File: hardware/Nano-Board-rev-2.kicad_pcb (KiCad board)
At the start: 2 copper layers, 125.7 x 53 mm, 75 parts, among them J1 Conn_01x02_Pin, J2 USB_B_Micro, J3 Conn_02x05_Odd_Even, J4 Conn_02x05_Odd_Even, J5 Conn_02x05_Odd_Even, J6 Micro_SD_Card_Det1, P1 Conn_02x05_Odd_Even, P2 Conn_02x05_Odd_Even, P3 Conn_02x05_Odd_Even, U1 STM32F303CCTx, U4 CDSOT236-0504C, U5 TLV75733PDBV, U6 STLINK-V3MODS, U8 MPU6050, Y1 8MHz Crystal

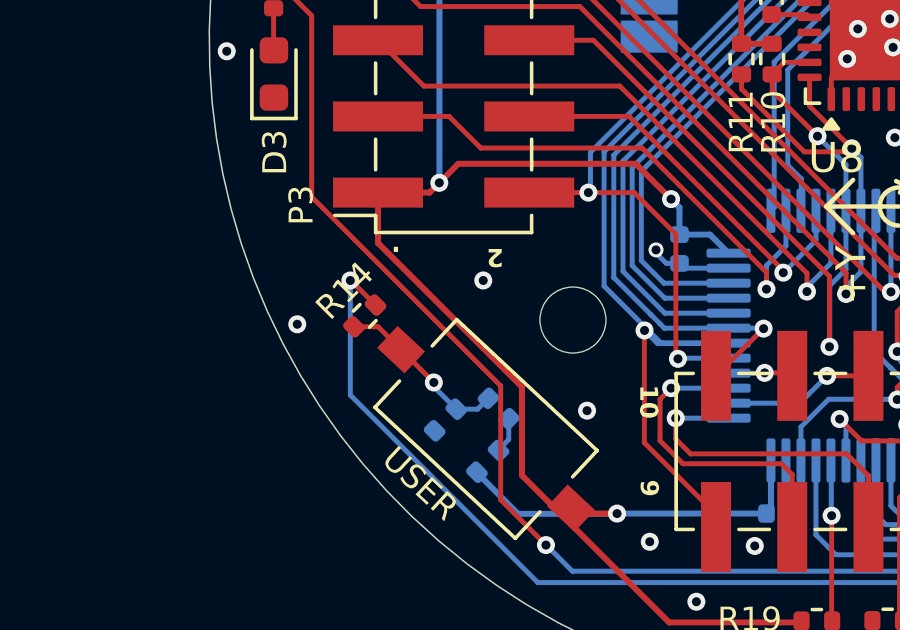
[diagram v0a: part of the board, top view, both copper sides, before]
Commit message: hardware: update PCB layout
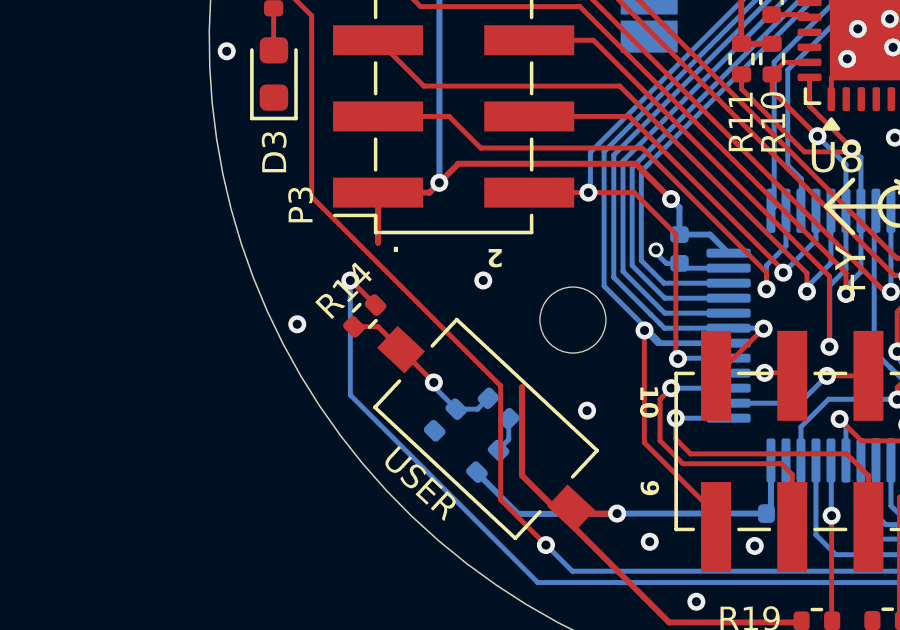
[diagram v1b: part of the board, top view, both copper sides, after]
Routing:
- net +3V3: track 190.4 -> 183.6 mm
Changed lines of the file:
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@@
-	)
-	(segment
-		(start 102.537308 108.456308)
-		(end 107.335 113.254)
-		(width 0.2)
-		(layer "F.Cu")
-		(net 2)
 	)
 	(segment

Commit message: hardware: update PCB layout
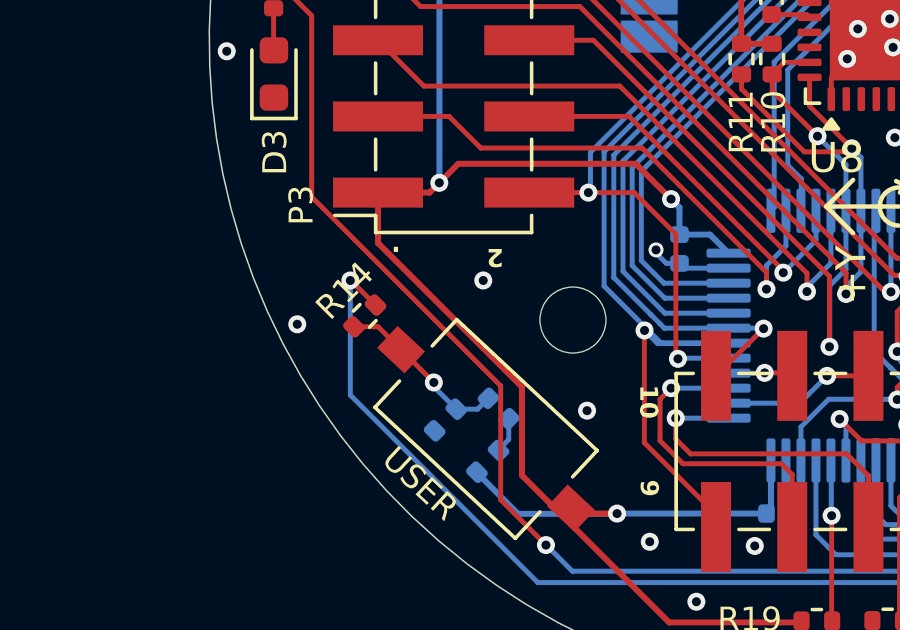
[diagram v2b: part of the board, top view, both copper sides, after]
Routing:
- net +3V3: track 183.6 -> 190.4 mm
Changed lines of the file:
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@@
+	)
+	(segment
+		(start 102.537308 108.456308)
+		(end 107.335 113.254)
+		(width 0.2)
+		(layer "F.Cu")
+		(net 2)
 	)
 	(segment
